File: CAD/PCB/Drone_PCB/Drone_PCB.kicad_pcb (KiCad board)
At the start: 2 copper layers, 85 x 50 mm, 73 parts, among them J1 MicroSD Holder, J10 UART1, J12 floor, J13 BATTERY, J14 ESC_POW1, J15 ESC_POW1, J16 ESC_POW1, J17 ESC_POW1, J2 MicroUSB Connector, J3 DEBUG, J4 CAM/SPI0, J5 ESP8266_WIFI, J6 M1, J7 M2, J8 M3, J9 M4, SW1 Button, SW2 Button, SW3 WiFi_RESET, SW4 UP, SW5 DOWN, U1 RP2040, U2 3V3 Regulator, U3 ICM-20948, U4 5V Regulator, U5 W25Q128JVSIQ TR, U6 Distance Sensor, U7 1V8 Regulator, Y1 12MHz

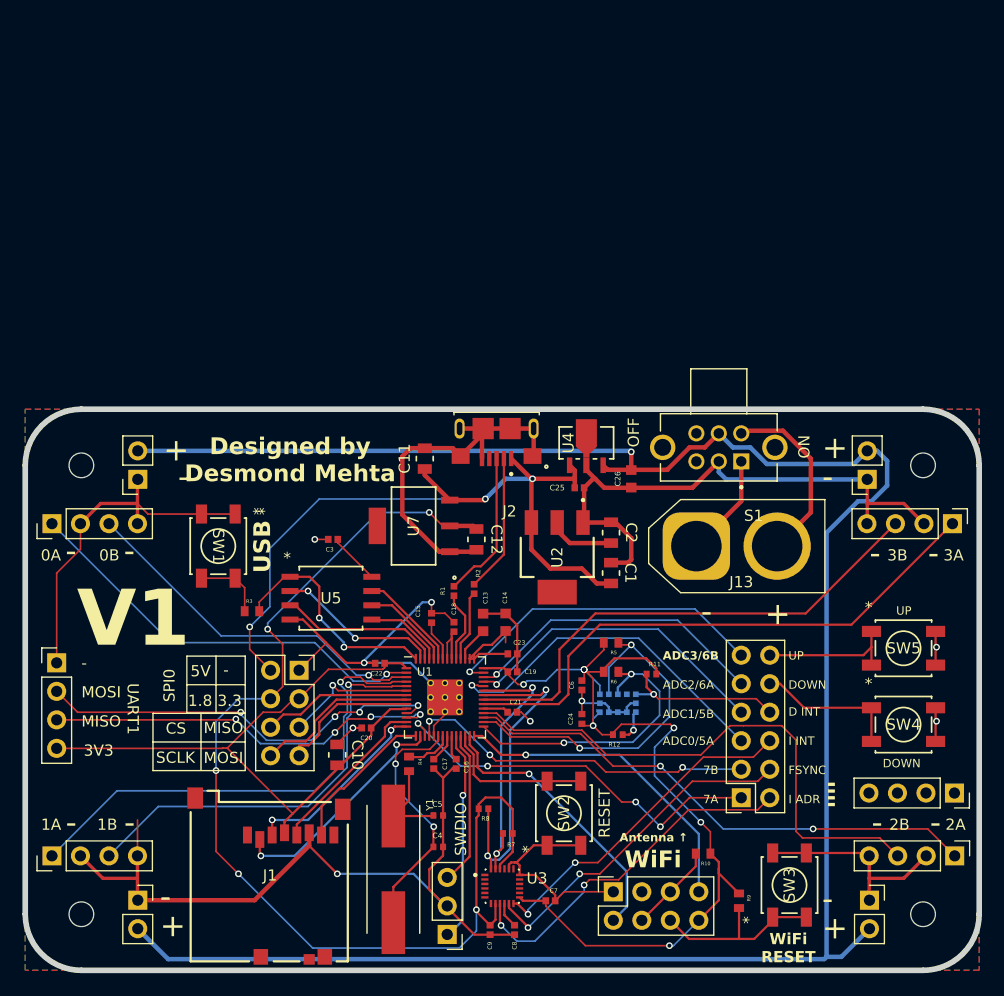
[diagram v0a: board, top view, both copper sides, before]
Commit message: pcb V2
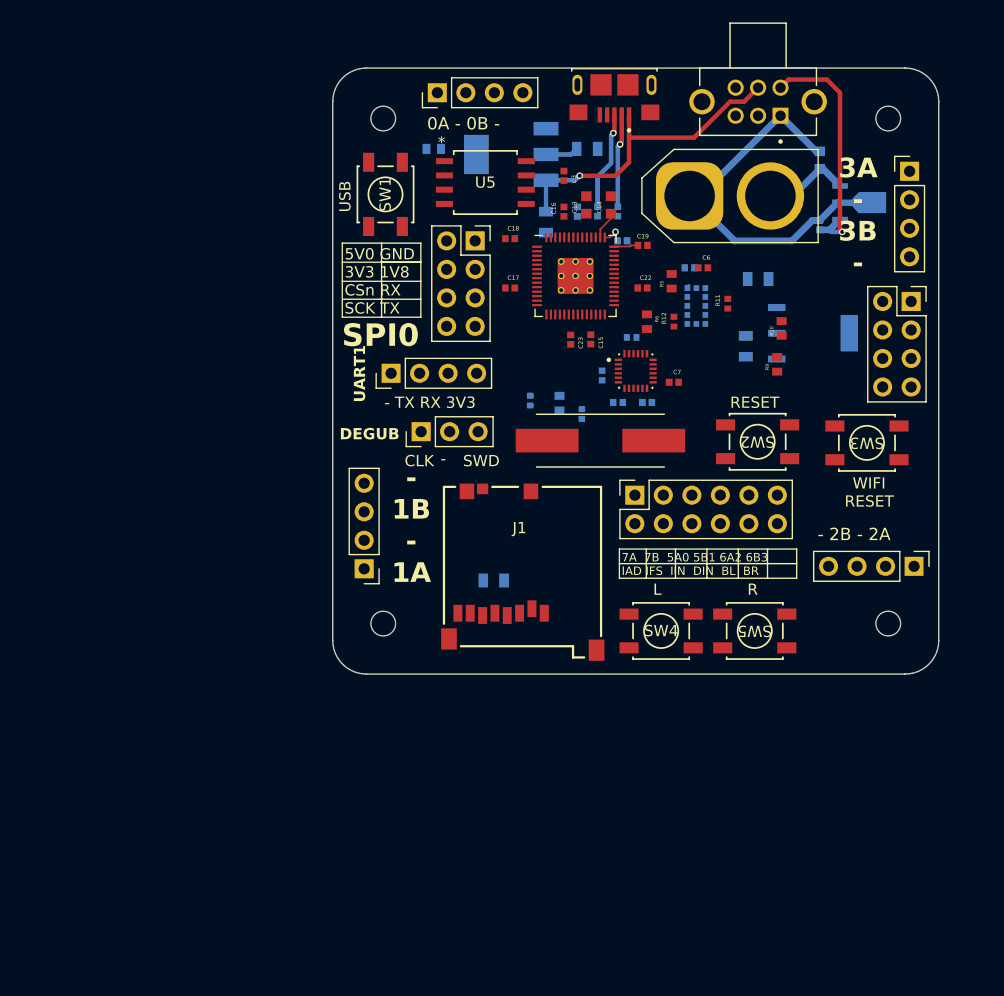
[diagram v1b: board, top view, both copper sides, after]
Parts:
- removed J12: floor, Connector_PinSocket_2.54mm:PinSocket_1x04_P2.54mm_Vertical
- removed J14, J15, J16, J17: ESC_POW1, Connector_PinSocket_2.54mm:PinSocket_1x02_P2.54mm_Vertical
- C1, C10, C11, C12, C2, C20, C21, C24, C25, C26, C4, C5, C8, C9, R1, R2, R3, R4, R7, R8, U2, U4, U7: moved to B.Cu
- moved H2 101.0 mm to (176.9, 74.1)
- moved J5 58.9 mm to (178.9, 90.4), turned to 0 degrees
- moved H4 54.6 mm to (131.9, 119.1)
- moved J6 51.5 mm to (136.7, 71.8)
- moved C16 50.1 mm to (148.0, 82.4), turned to 90 degrees
- moved C20 49.0 mm to (153.2, 85.0), turned to 0 degrees
- moved C8 48.5 mm to (155.4, 99.4), turned to 180 degrees
- moved C9 48.4 mm to (152.8, 99.4), turned to 0 degrees
- moved R9 47.9 mm to (167.0, 96.0), turned to 90 degrees
- moved C7 47.5 mm to (157.8, 97.6)
- moved U3 47.4 mm to (154.4, 96.6)
- moved R10 47.3 mm to (167.4, 92.8), turned to 90 degrees
- moved R7 45.6 mm to (154.0, 93.6)
- moved C21 45.0 mm to (149.2, 82.4), turned to 90 degrees
- moved J3 44.9 mm to (135.3, 102.0), turned to 90 degrees
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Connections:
- C25 pad 1: GND -> Net-(J13-Pin_1)
- C25 pad 2: +5V -> Net-(U4-VO)
- C26 pad 1: GND -> Net-(J13-Pin_1)
- C26 pad 2: Net-(J14-Pin_2) -> Net-(J13-Pin_2)
- S1 pad 4: Net-(J13-Pin_2) -> Net-(U4-VO)
- S1 pad 5: Net-(J14-Pin_2) -> +5V
- SW1 pad 2: Net-(R3-Pad1) -> GND
- SW1 pad 3: GND -> Net-(R3-Pad1)
- SW2 pad 2: Net-(U1-RUN) -> GND
- SW2 pad 3: GND -> Net-(U1-RUN)
- SW3 pad 1: Net-(J5-Pin_6) -> GND
- SW3 pad 4: GND -> Net-(J5-Pin_6)
- SW4 pad 2: GND -> Net-(J11-Pad10)
- SW4 pad 3: Net-(J11-Pad10) -> GND
- SW5 pad 1: Net-(J11-Pad12) -> GND
- SW5 pad 4: GND -> Net-(J11-Pad12)
- U4 pad 1: +5V -> Net-(U4-VO)
- U4 pad 2: GND -> Net-(J13-Pin_1)
- U4 pad 3: Net-(J14-Pin_2) -> Net-(J13-Pin_2)
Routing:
- net GND: track 286.9 -> 0.28 mm, vias 9 -> 0
- net Net-(J14-Pin_2): track 189.9 -> 0.00 mm, vias 1 -> 0
- net +3V3: track 172.6 -> 9.67 mm, vias 7 -> 1
- net +1V8: track 100.6 -> 0.00 mm, vias 5 -> 0
- net /M4_PWM_A: track 50.4 -> 0.00 mm
- net /M3_PWM_B: track 49.1 -> 0.00 mm
- net /M3_PWM_A: track 47.1 -> 0.00 mm, vias 2 -> 0
- net /M4_PWM_B: track 45.4 -> 0.00 mm
- net /M2_PWM_A: track 43.3 -> 0.00 mm, vias 1 -> 0
- net +5V: track 68.5 -> 28.4 mm, vias 3 -> 1
- net /M1_PWM_A: track 37.7 -> 0.00 mm, vias 1 -> 0
- net /M2_PWM_B: track 37.3 -> 0.00 mm, vias 1 -> 0
- net /UART1_TX: track 37.1 -> 0.00 mm, vias 4 -> 0
- net /UART1_RX: track 36.0 -> 0.00 mm, vias 4 -> 0
- net /PWM7A: track 35.0 -> 0.00 mm, vias 4 -> 0
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- removed copper zone on B.Cu, net GND
- removed copper zone on F.Cu, net GND
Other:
- board size 85 x 50 mm -> 54 x 54 mm
- board text added: "- 1B - 1A"
- board text added: "- 2B - 2A"
- board text added: "- TX RX 3V3"
- board text added: "0A - 0B -"
- board text added: "3A - 3B -"
- board text added: "5V0 GND 3V3 1V8 CSn RX SCK TX"
- board text added: "7A 7B 5A0 5B1 6A2 6B3 IAD IFS IIN DIN BL BR"
- board text added: "CLK"
- board text added: "DEGUB"
- board text added: "L"
- board text added: "R"
- board text added: "SWD"
- board text added: "WIFI RESET"
- board text removed: "+"
- board text removed: "0A"
- board text removed: "0B"
- board text removed: "1.8"
- board text removed: "1A"
- board text removed: "1B"
- board text removed: "2A"
- board text removed: "2B"
- board text removed: "3.3"
- board text removed: "3A"
- board text removed: "3B"
- board text removed: "3V3"
- board text removed: "5V"
- board text removed: "7A"
- board text removed: "7B"
- board text removed: "ADC0/5A"
- board text removed: "ADC1/5B"
- board text removed: "ADC2/6A"
- board text removed: "ADC3/6B"
- board text removed: "Antenna ↑"
- board text removed: "CS"
- board text removed: "D INT"
- board text removed: "DOWN"
- board text removed: "Designed by Desmond Mehta"
- board text removed: "FSYNC"
- board text removed: "I ADR"
- board text removed: "I INT"
- board text removed: "MISO"
- board text removed: "MOSI"
- board text removed: "OFF"
- board text removed: "ON"
- board text removed: "SCLK"
- board text removed: "SWDIO"
- board text removed: "UP"
- board text removed: "V1"
- board text removed: "WiFi"
- board text removed: "WiFi RESET"
